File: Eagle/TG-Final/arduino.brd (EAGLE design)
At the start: 172.7 x 76.2 mm, 4 parts

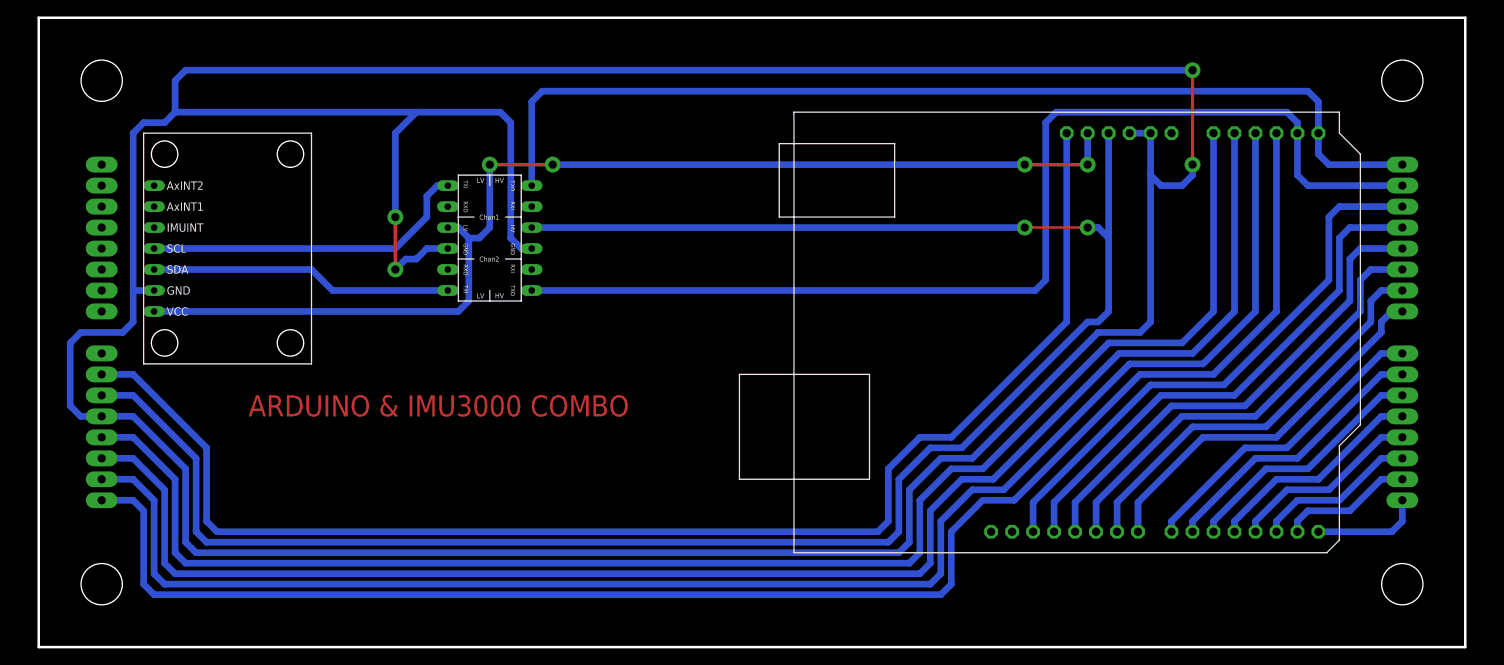
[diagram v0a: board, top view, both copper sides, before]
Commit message: Muchos Cambios a 2 dias de la denfesa
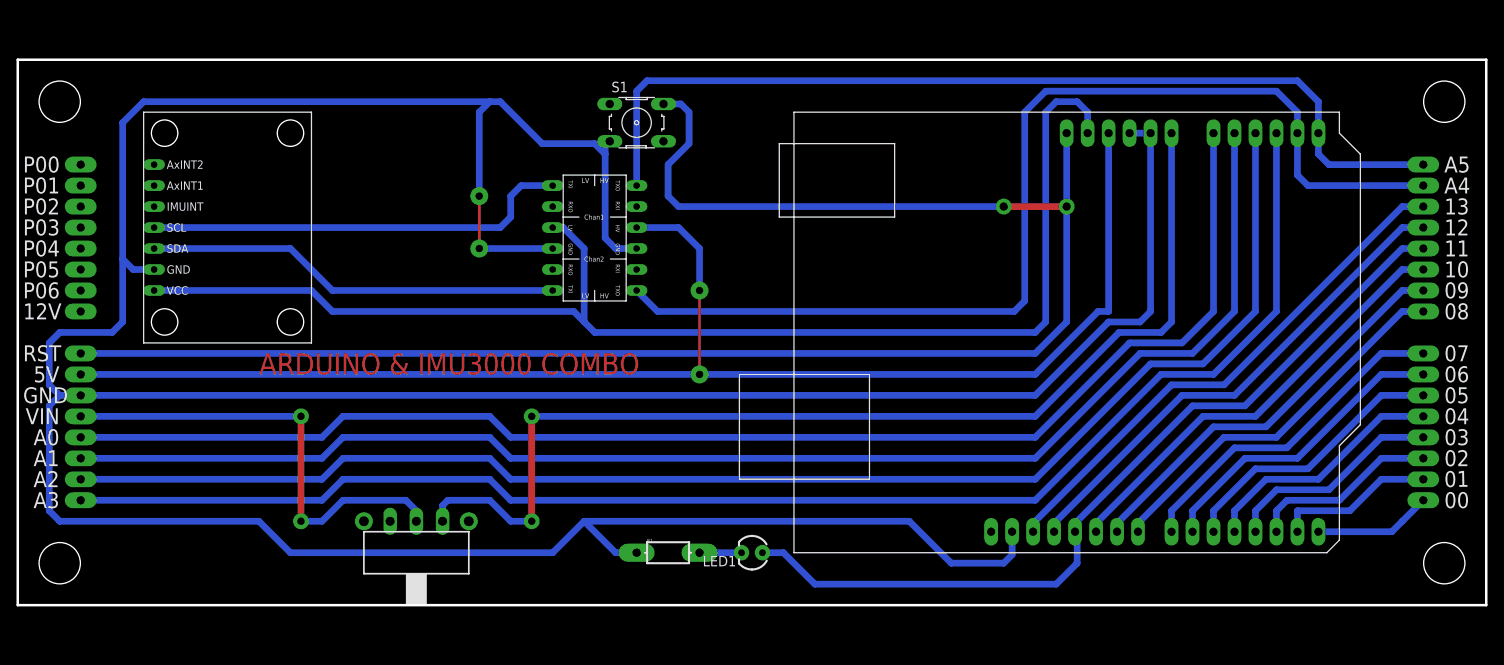
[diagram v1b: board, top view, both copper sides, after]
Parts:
- added LED1: (no value), SparkFun:LED3MM
- added R1: (no value), SparkFun:AXIAL-0.3-KIT
- added S1: (no value), switch-omron:B3F-10XX
- added S2: TL39YOSWITCH_2_ESTADOS, aasanchez:TL3XYO
- U$1: value BASEFINAL -> BASE-FINAL
- moved U$8 12.7 mm to (-128.3, 67.3)
- moved U$7 2.54 mm to (-179.1, 62.2)
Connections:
- removed net PIN09: U$1.P$10, U$6.RESET
- removed net PIN10: U$1.P$11, U$6.5V, U$8.P$10
- removed net PIN11: U$1.P$12, U$6.GND1, U$6.GND2, U$7.VSS, U$8.P$4, U$8.P$9
- removed net PIN12: U$1.P$13, U$6.A0
- removed net PIN13: U$1.P$14, U$6.A1
- removed net PIN14: U$1.P$15, U$6.A2
- removed net PIN15: U$1.P$16, U$6.A3
- removed net PIN30: U$1.P$31, U$6.A4, U$8.P$7
- removed net PIN31: U$1.P$32, U$6.A5, U$8.P$12
- new net 5V: U$1.5V, U$6.5V, U$8.P$10
- new net A0: U$1.A0, U$6.A0
- new net A1: U$1.A1, U$6.A1
- new net A2: U$1.A2, U$6.A2
- new net A3: U$1.A3, U$6.A3
- new net A4: U$1.A4, U$6.A4, U$8.P$7
- new net A5: U$1.A5, U$6.A5, U$8.P$12
- new net N$4: S2.2, U$1.VIN
- new net N$5: LED1.K, R1.P$2
- new net RST: S1.2, U$1.RST, U$6.RESET
- net GND: now also R1.P$1, S1.3, U$1.GND, U$6.GND1, U$6.GND2, U$7.VSS, U$8.P$4, U$8.P$9
- net PIN16: now also U$1.0; no longer U$1.P$17
- net PIN17: now also U$1.1; no longer U$1.P$18
- net PIN18: now also U$1.2; no longer U$1.P$19
- net PIN19: now also U$1.3; no longer U$1.P$20
- net PIN20: now also U$1.4; no longer U$1.P$21
- net PIN21: now also U$1.5; no longer U$1.P$22
- net PIN22: now also U$1.6; no longer U$1.P$23
- net PIN23: now also U$1.7; no longer U$1.P$24
- net PIN24: now also U$1.8; no longer U$1.P$25
- net PIN25: now also U$1.9; no longer U$1.P$26
- net PIN26: now also U$1.10; no longer U$1.P$27
- net PIN27: now also LED1.A, U$1.11; no longer U$1.P$28
- net PIN28: now also U$1.12; no longer U$1.P$29
- net PIN29: now also U$1.13; no longer U$1.P$30
- net VIN: now also S2.1
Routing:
- net PIN11: track 464.0 -> 0.00 mm, vias 4 -> 0
- net GND: track 0.00 -> 459.6 mm, vias 0 -> 2
- net PIN10: track 241.8 -> 0.00 mm, vias 2 -> 0
- net RST: track 0.00 -> 207.3 mm, vias 0 -> 2
- net PIN15: track 191.7 -> 0.00 mm
- net PIN14: track 189.2 -> 0.00 mm
- net PIN13: track 186.6 -> 0.00 mm
- net PIN12: track 184.1 -> 0.00 mm
- net A3: track 0.00 -> 177.9 mm
- net A2: track 0.00 -> 174.4 mm
- net 5V: track 0.00 -> 173.1 mm, vias 0 -> 2
- net A1: track 0.00 -> 170.8 mm
- net A0: track 0.00 -> 167.2 mm
- net PIN09: track 167.0 -> 0.00 mm
- net PIN30: track 132.9 -> 0.00 mm
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- added copper zone on layer 16, net N$3
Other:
- board size 172.7 x 76.2 mm -> 177.8 x 66 mm
